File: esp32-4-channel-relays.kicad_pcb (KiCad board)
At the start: 2 copper layers, 86.4 x 86.6 mm, 63 parts, among them J1 Relay-1, J2 Relay-2, J3 Relay-3, J4 Relay-4, K1 SRD-05VDC-SL-C, K2 SRD-05VDC-SL-C, K3 SRD-05VDC-SL-C, K4 SRD-05VDC-SL-C, Q1 MBT3904DW1, Q2 BC547A, Q3 BC547A, Q4 BC547A, Q5 BC547A, SW1 SW_SKQG, SW2 SW_SKQG, U1 AMS1117-3.3, U2 CH340C, U3 PRTR5V0U2X, U4 ESP32-WROOM-32, U5 PC817, U6 PC817, U7 PC817, U8 PC817

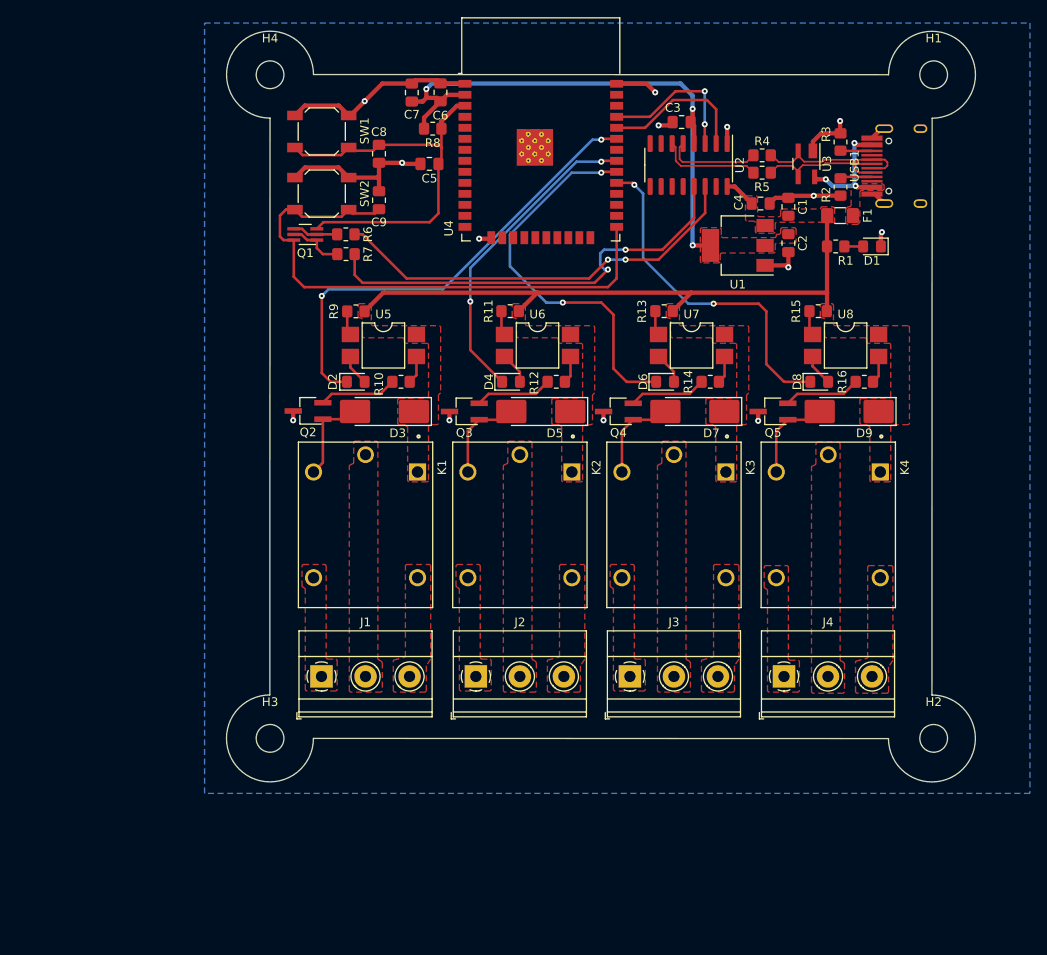
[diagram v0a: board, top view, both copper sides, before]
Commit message: Design rules check and lock components
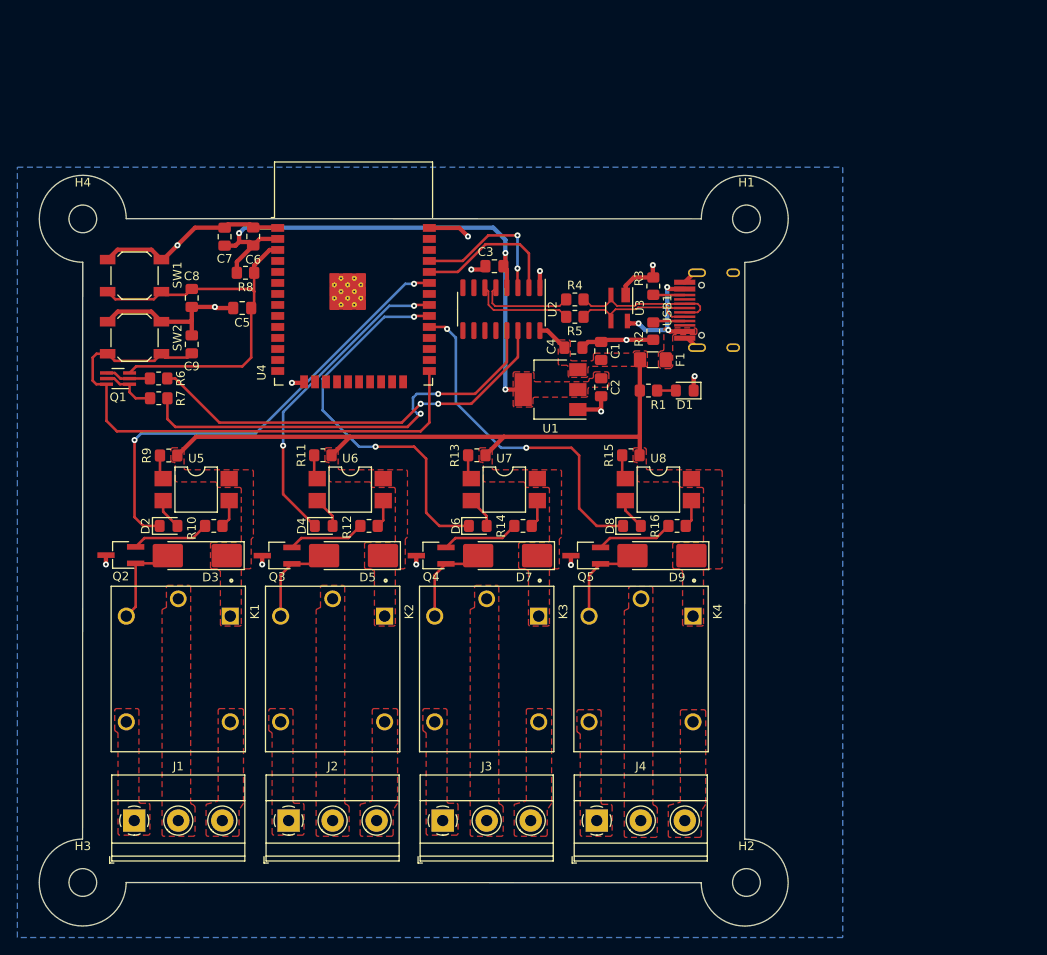
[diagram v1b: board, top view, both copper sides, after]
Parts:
- moved R16 27.3 mm to (173.6, 105.7)
- moved C9 27.3 mm to (117.6, 84.7)
- moved R6 27.3 mm to (113.8, 88.6)
- moved R7 27.3 mm to (113.8, 90.9)
- moved R9 27.3 mm to (114.9, 97.5)
- moved C7 27.3 mm to (121.4, 72.3)
- moved C8 27.3 mm to (117.6, 79.3)
- moved J1 27.3 mm to (110.9, 139.7)
- moved R3 27.3 mm to (170.8, 78.0)
- moved C1 27.3 mm to (164.8, 85.5)
- moved C4 27.3 mm to (161.6, 85.1)
- moved D2 27.3 mm to (114.9, 105.7)
- moved D3 27.3 mm to (118.2, 109.1)
- moved D4 27.3 mm to (132.8, 105.7)
- moved D5 27.3 mm to (136.3, 109.1)
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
